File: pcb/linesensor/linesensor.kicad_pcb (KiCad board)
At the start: 2 copper layers, 20.8 x 18.6 mm, 4 parts, among them J1 Conn_01x03_Socket, U1 TRCT5000

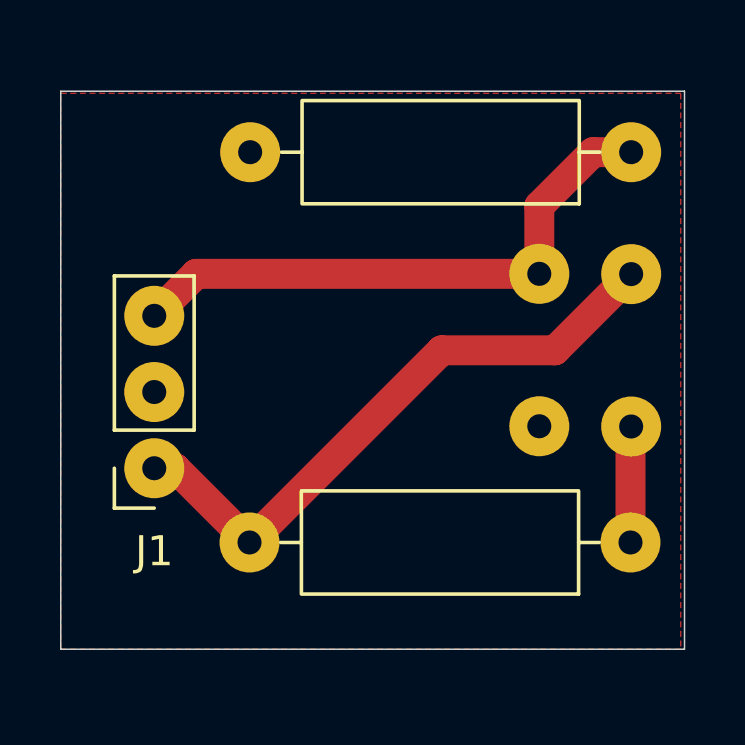
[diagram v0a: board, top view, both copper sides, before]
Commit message: init
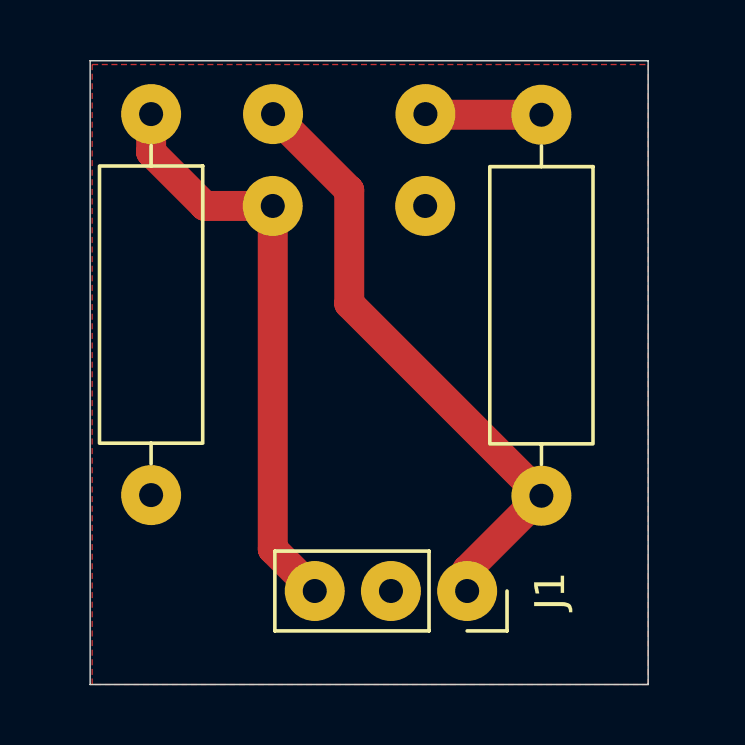
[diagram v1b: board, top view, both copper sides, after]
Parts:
- moved R2 16.1 mm to (32.5, 26.2), turned to -90 degrees
- moved R1 14.6 mm to (45.5, 26.2), turned to -90 degrees
- moved J1 11.2 mm to (43.0, 42.1), turned to -90 degrees
- moved U1 7.96 mm to (39.1, 29.2), turned to -90 degrees
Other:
- board size 20.8 x 18.6 mm -> 18.6 x 20.8 mm
